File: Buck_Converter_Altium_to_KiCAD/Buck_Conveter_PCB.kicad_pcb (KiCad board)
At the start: 4 copper layers, 101.6 x 50.8 mm, 23 parts, among them J1 XT30, J2 XT30, U1 LM61495RPHR

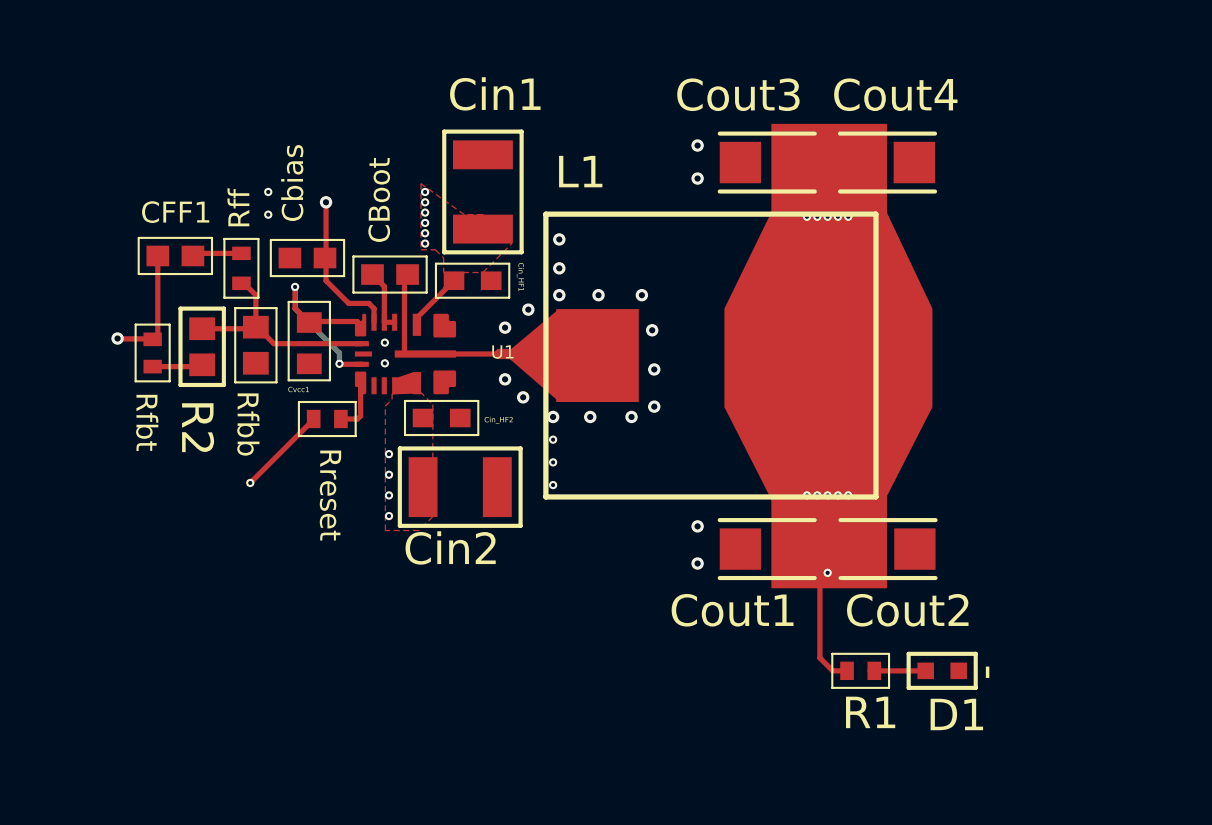
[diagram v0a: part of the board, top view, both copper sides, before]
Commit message: Updated PCB
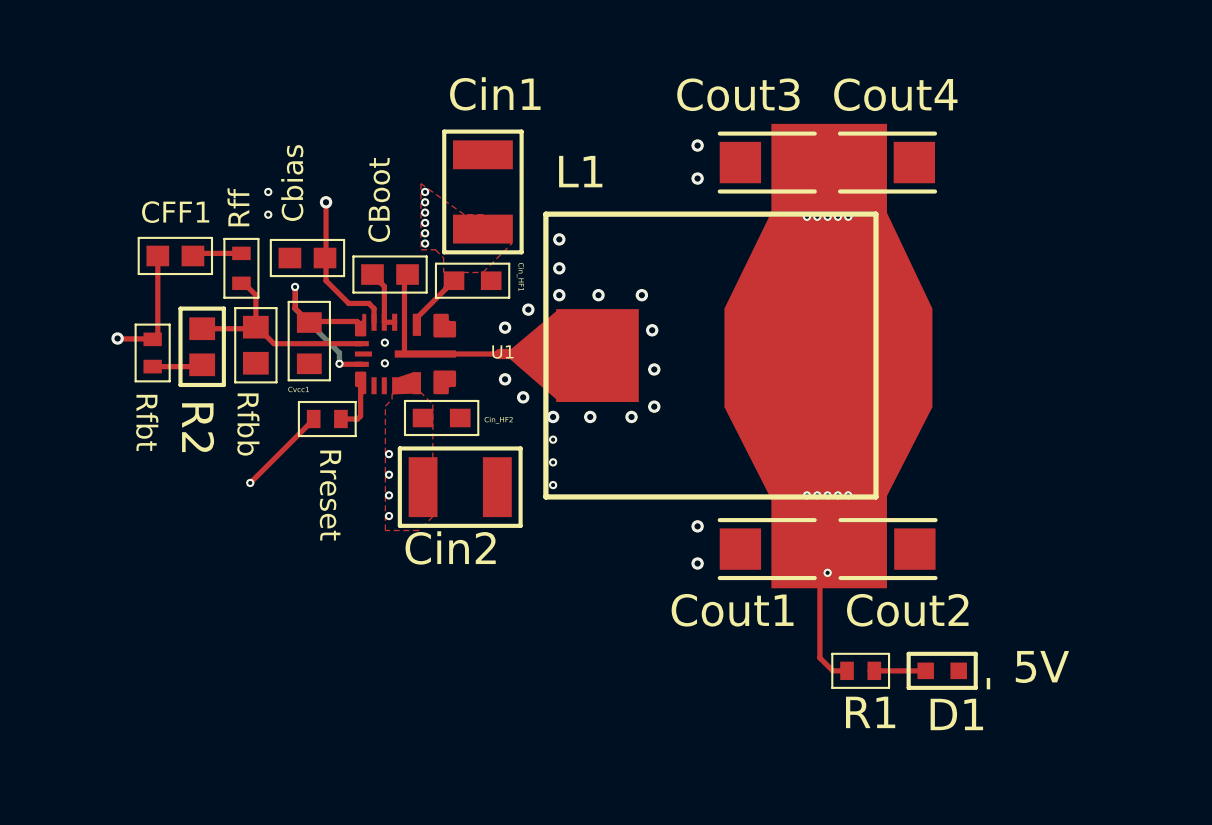
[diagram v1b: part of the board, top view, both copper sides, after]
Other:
- board text added: "5V"
